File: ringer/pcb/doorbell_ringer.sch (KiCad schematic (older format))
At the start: 13 parts, among them U2 TL074

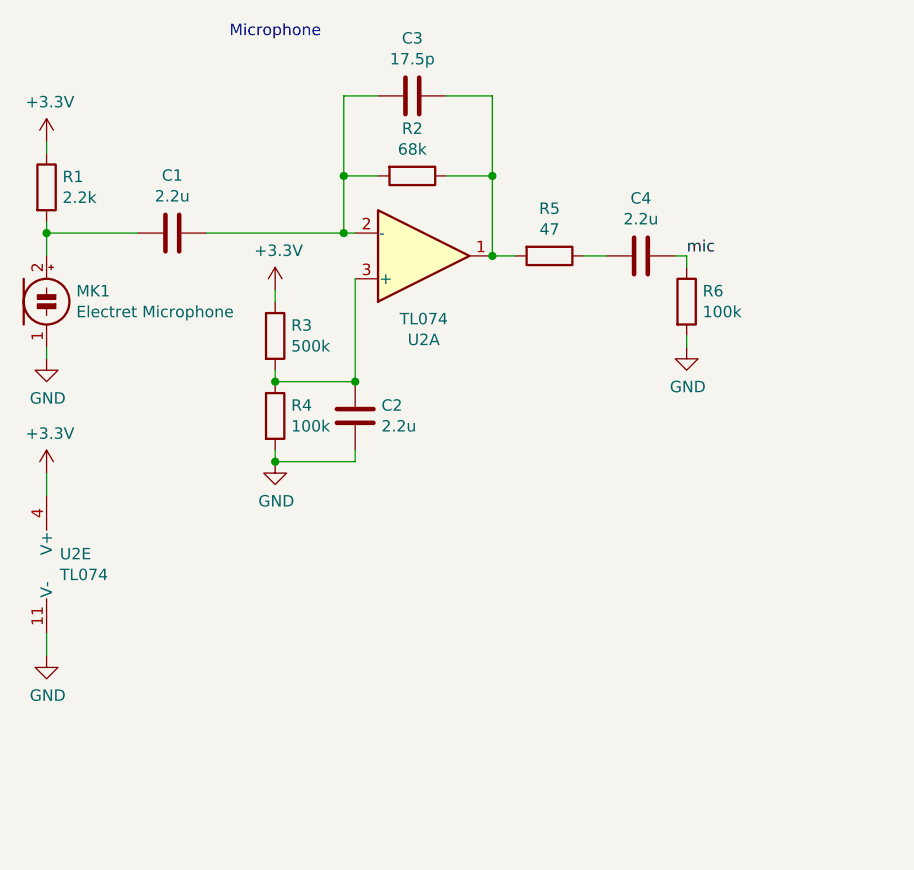
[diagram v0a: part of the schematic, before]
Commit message: Mic Pre amp
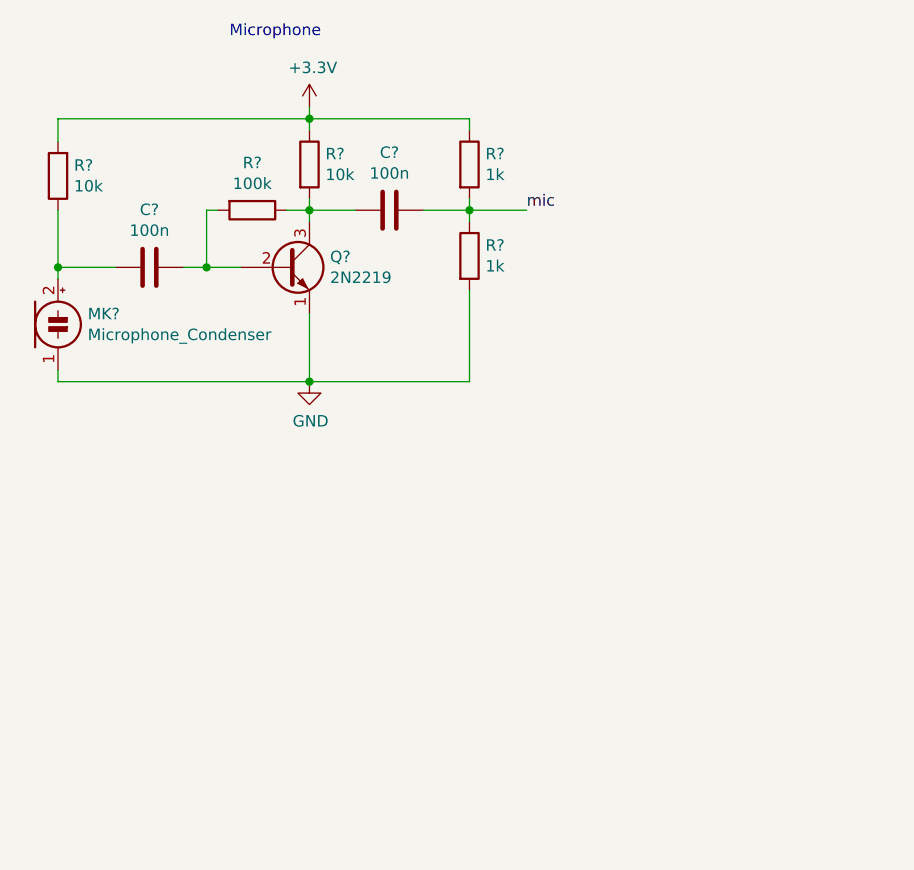
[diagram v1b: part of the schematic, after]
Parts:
- removed C1, C2, C4: 2.2u, symbol Device:C
- removed C3: 17.5p, symbol Device:C
- removed MK1: Electret Microphone, symbol Device:Microphone_Condenser
- removed R1: 2.2k, symbol Device:R
- removed R2: 68k, symbol Device:R
- removed R3: 500k, symbol Device:R
- removed R4, R6: 100k, symbol Device:R
- removed R5: 47, symbol Device:R
- removed U2: TL074, symbol Amplifier_Operational:TL074
- added C? (x2): 100n, symbol Device:C
- added MK?: Microphone_Condenser, symbol Device:Microphone_Condenser
- added Q?: 2N2219, Package_TO_SOT_THT:TO-39-3, symbol Transistor_BJT:2N2219
- added R? (x2): 10k, symbol Device:R
- added R?: 100k, symbol Device:R
- added R? (x2): 1k, symbol Device:R
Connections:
- net +3V3: now also R?.1, R?.1, R?.2
- net GND: now also MK?.1 (-), Q?.1 (E), R?.2
- net mic: now also C?.1, R?.1, R?.2
- new net: C?.1, Q?.2 (B), R?.2
- new net: C?.2, Q?.3 (C), R?.1, R?.2
- new net: C?.2, MK?.2 (+), R?.1
